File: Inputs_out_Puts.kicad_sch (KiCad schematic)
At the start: 29 parts, among them J3 Conn_01x01, J4 Conn_01x02_Female, J5 Conn_01x04_Female, J6 Conn_01x04_Female, J8 Conn_01x01, J9 Conn_01x01, SW1 SW_MEC_5G, U1 TCAN330

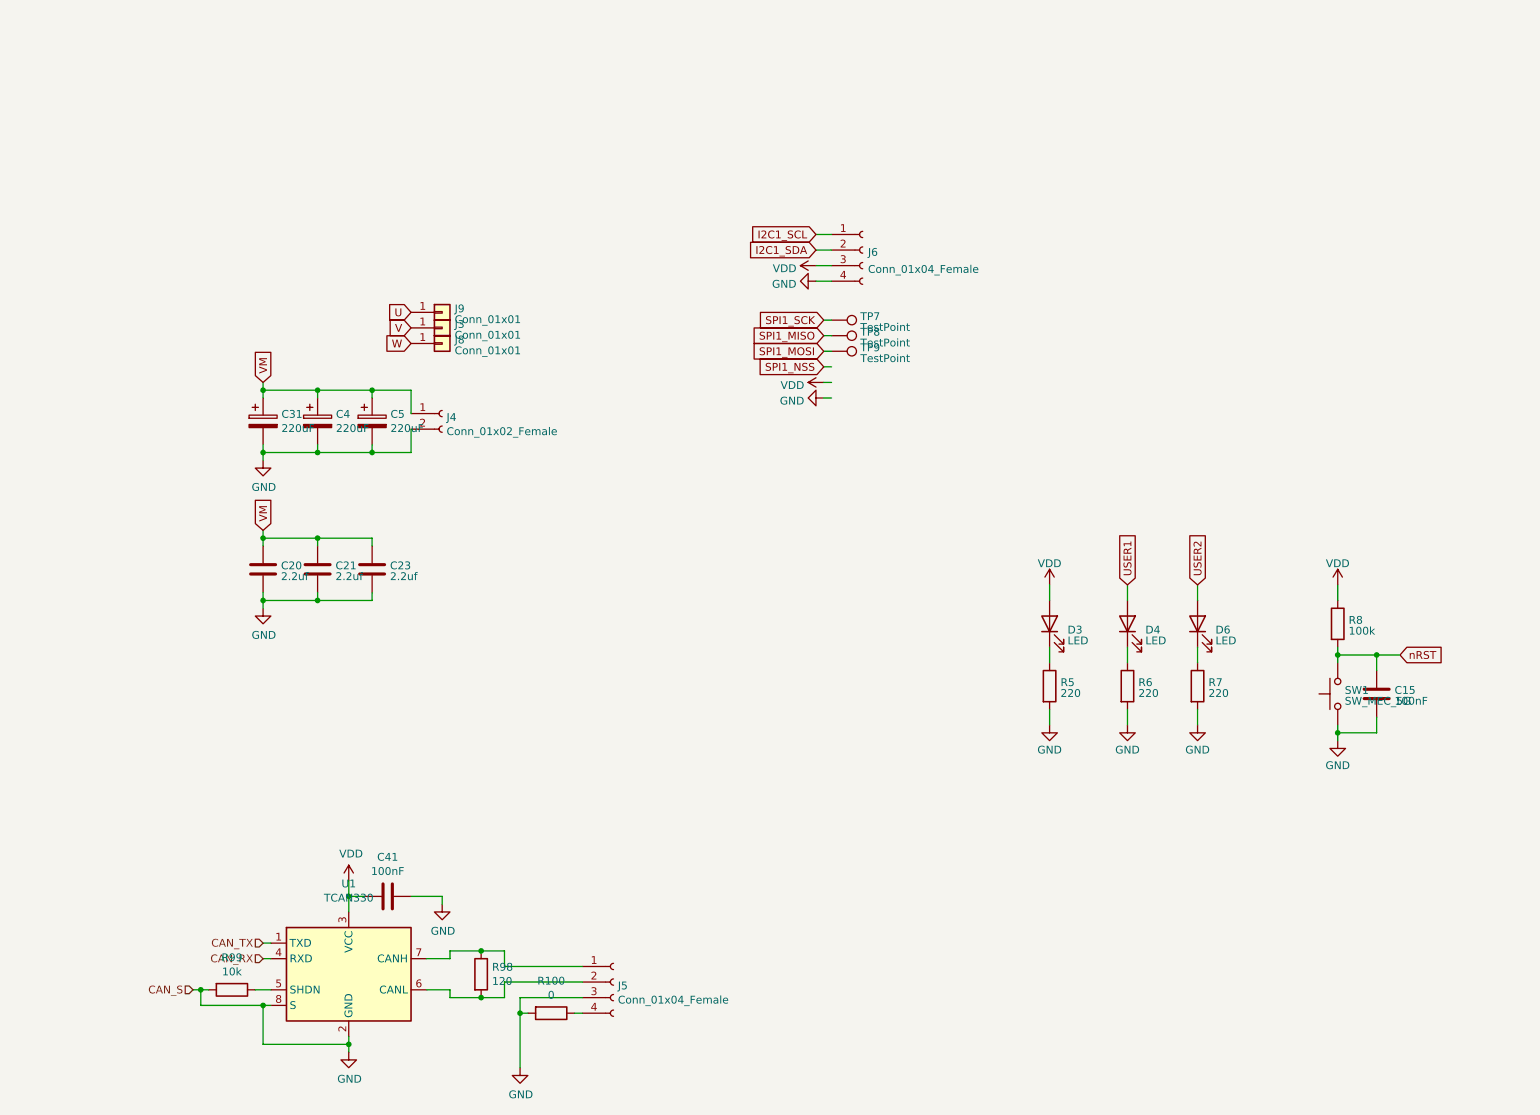
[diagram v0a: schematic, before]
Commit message: Can't remember what these changes are
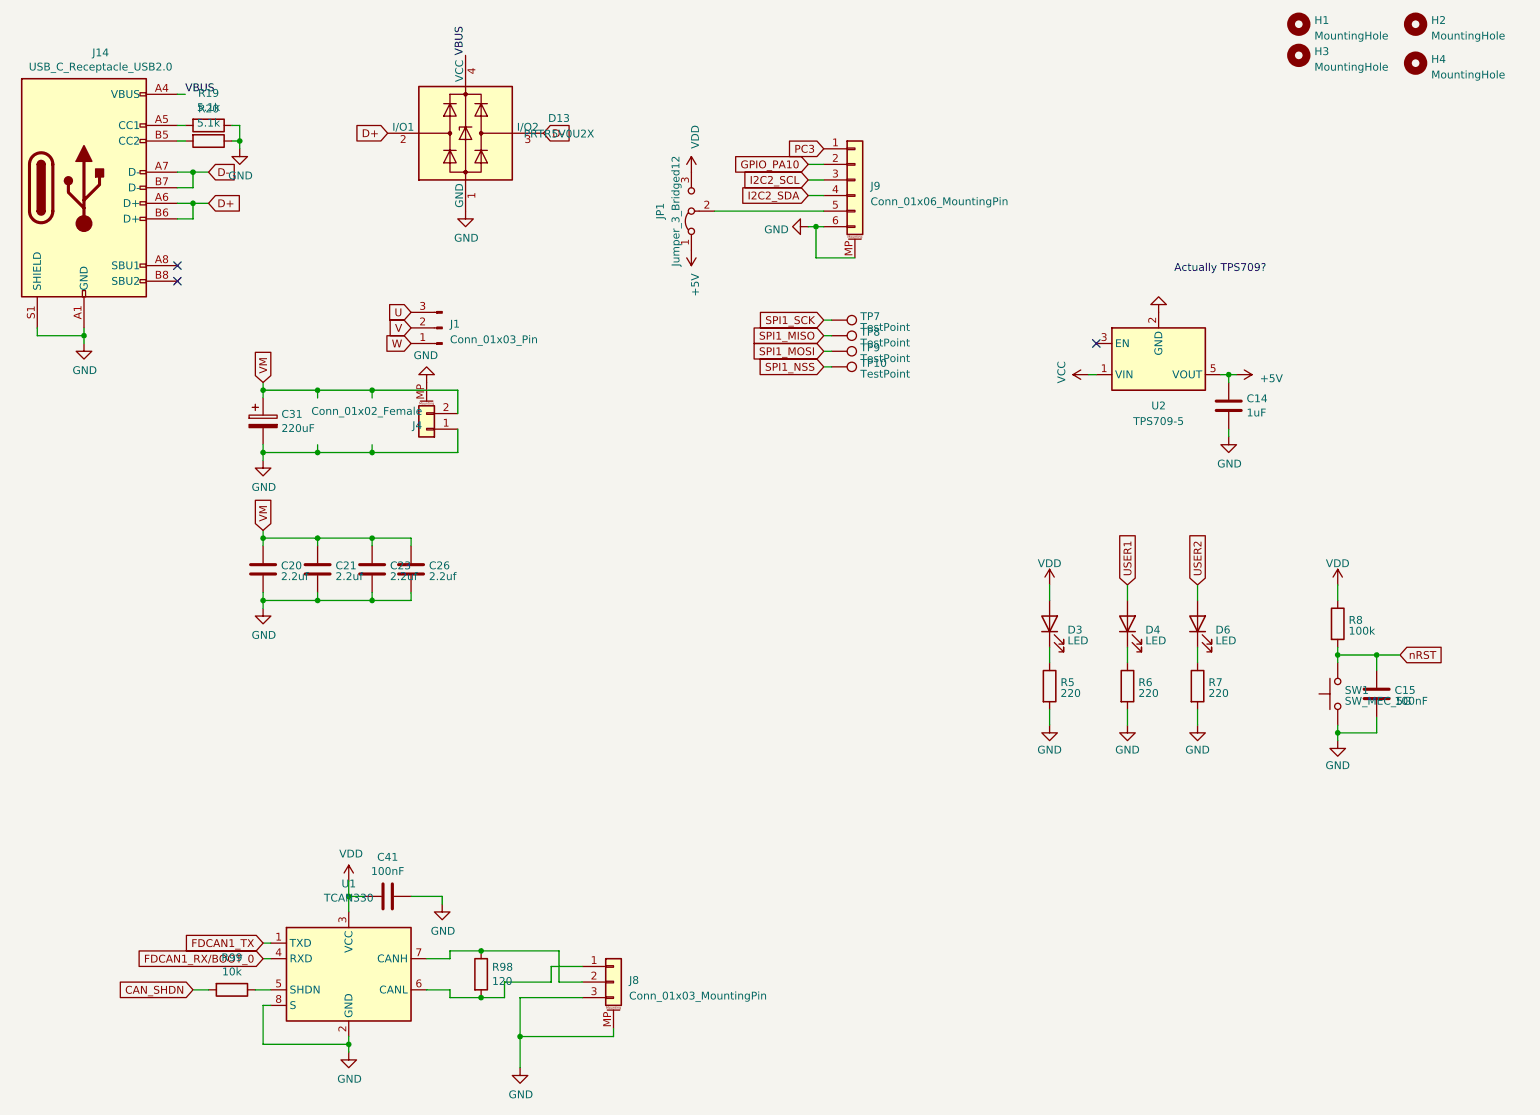
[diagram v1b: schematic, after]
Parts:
- removed C4, C5: 220uF, Capacitor_SMD:CP_Elec_8x10, symbol Device:CP
- removed J3, J8, J9: Conn_01x01, my_stuff:connector_wire_esc, symbol Connector_Generic:Conn_01x01
- removed J5: Conn_01x04_Female, Connector_PinSocket_2.54mm:PinSocket_1x04_P2.54mm_Vertical, symbol Connector:Conn_01x04_Female
- removed J6: Conn_01x04_Female, Connector_PinHeader_2.54mm:PinHeader_1x04_P2.54mm_Vertical, symbol Connector:Conn_01x04_Female
- removed R100: 0, Resistor_SMD:R_0603_1608Metric, symbol Device:R
- added C14: 1uF, Capacitor_SMD:C_0603_1608Metric, symbol Device:C
- added C26: 2.2uf, Capacitor_SMD:C_1206_3216Metric, symbol Device:C
- added D13: PRTR5V0U2X, Package_TO_SOT_SMD:SOT-143, symbol Power_Protection:PRTR5V0U2X
- added H1, H2, H3, H4: MountingHole, MountingHole:MountingHole_3.2mm_M3_ISO14580, symbol Mechanical:MountingHole
- added J1: Conn_01x03_Pin, mystuff:flat_3, symbol Connector:Conn_01x03_Pin
- added J14: USB_C_Receptacle_USB2.0, Connector_USB:USB_C_Receptacle_XKB_U262-16XN-4BVC11, symbol Connector:USB_C_Receptacle_USB2.0
- added J8: Conn_01x03_MountingPin, Connector_JST:JST_SH_BM03B-SRSS-TB_1x03-1MP_P1.00mm_Vertical, symbol Connector_Generic_MountingPin:Conn_01x03_MountingPin
- added J9: Conn_01x06_MountingPin, Connector_JST:JST_SH_BM06B-SRSS-TB_1x06-1MP_P1.00mm_Vertical, symbol Connector_Generic_MountingPin:Conn_01x06_MountingPin
- added JP1: Jumper_3_Bridged12, Jumper:SolderJumper-3_P1.3mm_Bridged2Bar12_RoundedPad1.0x1.5mm_NumberLabels, symbol Jumper:Jumper_3_Bridged12
- added R19, R20: 5.1k, Resistor_SMD:R_0603_1608Metric, symbol Device:R
- added TP10: TestPoint, TestPoint:TestPoint_Pad_D1.5mm, symbol Connector:TestPoint
- added U2: TPS709-5, Package_TO_SOT_SMD:TSOT-23-5, symbol mystuff:TPS709-5
- J4: footprint Connector_AMASS:AMASS_XT60-F_1x02_P7.20mm_Vertical -> Connector_AMASS:AMASS_XT30PW-M_1x02_P2.50mm_Horizontal; symbol Connector:Conn_01x02_Female -> Connector_Generic_MountingPin:Conn_01x02_MountingPin
- SW1: footprint Button_Switch_SMD:SW_SPST_PTS810 -> mystuff:SW_SPST_TS-1187A-B; LCSC (none) -> C318884
- TP7, TP8, TP9: footprint TestPoint:TestPoint_Pad_D1.5mm -> TestPoint:TestPoint_Pad_D1.0mm
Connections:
- net GND: now also J4.1 (Pin_1), J4.MP (MountPin), C14.2, C26.2, D13.1 (GND), J14.A1 (GND), J14.A12 (GND), J14.B1 (GND), J14.B12 (GND), J14.S1 (SHIELD), J8.3 (Pin_3), J8.MP (MountPin), J9.6 (Pin_6), J9.MP (MountPin), R19.1, R20.1, U2.2 (GND); no longer J4.2 (Pin_2), R99.2
- net SPI1_NSS: now also TP10.1
- net U: now also J1.3 (Pin_3)
- net V: now also J1.2 (Pin_2)
- net VDD: now also JP1.3 (B)
- net VM: now also J4.2 (Pin_2), C26.1; no longer J4.1 (Pin_1)
- net W: now also J1.1 (Pin_1)
- net at R98.2, U1.6 (CANL): now also J8.1 (Pin_1)
- net at R98.1, U1.7 (CANH): now also J8.2 (Pin_2)
- net CAN_RX renamed FDCAN1_RX/BOOT_0
- net CAN_TX renamed FDCAN1_TX
- new net: J14.B5 (CC2), R20.2
- new net: J14.A5 (CC1), R19.2
- new net: J9.5 (Pin_5), JP1.2 (C)
- new net +5V: C14.1, JP1.1 (A), U2.5 (VOUT)
- new net CAN_SHDN: R99.2
- new net D+: D13.2 (I/O1), J14.A6 (D+), J14.B6 (D+)
- new net D-: D13.3 (I/O2), J14.A7 (D-), J14.B7 (D-)
- new net GPIO_PA10: J9.2 (Pin_2)
- new net I2C2_SCL: J9.3 (Pin_3)
- new net I2C2_SDA: J9.4 (Pin_4)
- new net PC3: J9.1 (Pin_1)
- new net VBUS: D13.4 (VCC), J14.A4 (VBUS), J14.A9 (VBUS), J14.B4 (VBUS), J14.B9 (VBUS)
- new net VCC: U2.1 (VIN)
- no-connect marks 0 -> 3
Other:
- note added: "Actually TPS709?"

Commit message: revision 3
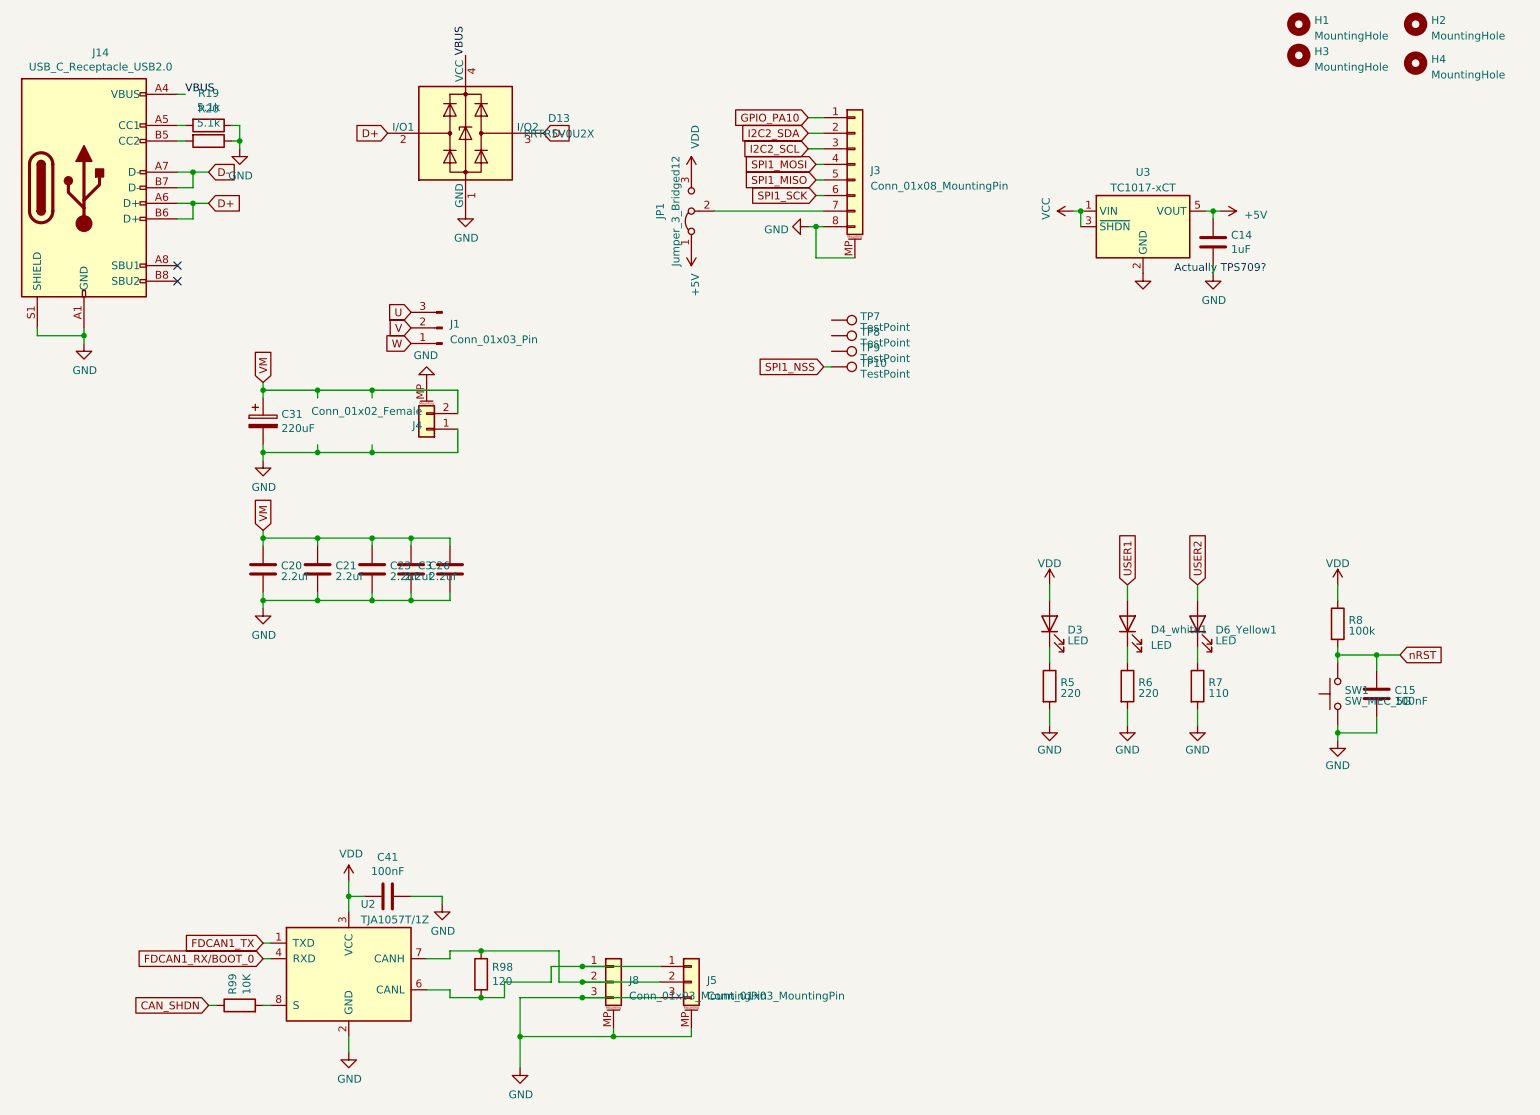
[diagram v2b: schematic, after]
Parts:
- removed J9: Conn_01x06_MountingPin, Connector_JST:JST_SH_BM06B-SRSS-TB_1x06-1MP_P1.00mm_Vertical, symbol Connector_Generic_MountingPin:Conn_01x06_MountingPin
- removed U1: TCAN330, Package_SO:SOIC-8_3.9x4.9mm_P1.27mm, symbol Interface_CAN_LIN:TCAN330
- removed U2: TPS709-5, Package_TO_SOT_SMD:TSOT-23-5, symbol mystuff:TPS709-5
- added C3: 2.2uf, Capacitor_SMD:C_1206_3216Metric, symbol Device:C
- added J3: Conn_01x08_MountingPin, Connector_JST:JST_SH_BM08B-SRSS-TB_1x08-1MP_P1.00mm_Vertical, symbol Connector_Generic_MountingPin:Conn_01x08_MountingPin
- added J5: Conn_01x03_MountingPin, Connector_JST:JST_SH_BM03B-SRSS-TB_1x03-1MP_P1.00mm_Vertical, symbol Connector_Generic_MountingPin:Conn_01x03_MountingPin
- added U2: TJA1057T/1Z, Package_SO:SOIC-8_3.9x4.9mm_P1.27mm, symbol Interface_CAN_LIN:TJA1051T
- added U3: TC1017-xCT, Package_TO_SOT_SMD:SOT-23-5, symbol Regulator_Linear:TC1017-xCT
- C14: footprint Capacitor_SMD:C_0603_1608Metric -> Capacitor_SMD:C_0402_1005Metric; LCSC Part C15849 -> (none)
- C15, C41: footprint Capacitor_SMD:C_0603_1608Metric -> Capacitor_SMD:C_0402_1005Metric
- R19: footprint Resistor_SMD:R_0603_1608Metric -> Resistor_SMD:R_0402_1005Metric; LCSC Part C23186 -> (none)
- R20, R5, R6, R8, R98: footprint Resistor_SMD:R_0603_1608Metric -> Resistor_SMD:R_0402_1005Metric
- R7: value 220 -> 110; footprint Resistor_SMD:R_0603_1608Metric -> Resistor_SMD:R_0402_1005Metric
- R99: value 10k -> 10K; footprint Resistor_SMD:R_0603_1608Metric -> Resistor_SMD:R_0402_1005Metric
- renumbered D4 to D4_white1, D6 to D6_Yellow1
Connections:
- net +5V: now also U3.5 (VOUT)
- net CAN_SHDN: now also R99.1; no longer R99.2
- net FDCAN1_RX/BOOT_0: now also U2.4 (RXD)
- net FDCAN1_TX: now also U2.1 (TXD)
- net GND: now also C3.2, J3.8 (Pin_8), J3.MP (MountPin), J5.3 (Pin_3), J5.MP (MountPin), U2.2 (GND), U3.2 (GND)
- net GPIO_PA10: now also J3.1 (Pin_1)
- net I2C2_SCL: now also J3.3 (Pin_3)
- net I2C2_SDA: now also J3.2 (Pin_2)
- net SPI1_MISO: now also J3.5 (Pin_5); no longer TP8.1
- net SPI1_MOSI: now also J3.4 (Pin_4); no longer TP9.1
- net SPI1_SCK: now also J3.6 (Pin_6); no longer TP7.1
- net VCC: now also U3.1 (VIN), U3.3 (~{SHDN})
- net VDD: now also U2.3 (VCC)
- net VM: now also C3.1
- net at J8.1 (Pin_1), R98.2: now also J5.1 (Pin_1), U2.6 (CANL)
- net at J8.2 (Pin_2), R98.1: now also J5.2 (Pin_2), U2.7 (CANH)
- net at JP1.2 (C): now also J3.7 (Pin_7)
- new net: R99.2, U2.8 (S)
- no-connect marks 3 -> 2
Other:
- moved on the sheet: C14
